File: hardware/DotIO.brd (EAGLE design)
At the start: 30 x 65 mm, 37 parts, among them CN1 1X4-BIG, U1 ATMEGA328P-MU-QFN32, X1 S4B-ZR, X2 S4B-ZR, X3 S4B-ZR, X4 S4B-ZR, X5 S4B-ZR, X6 S4B-ZR, X7 S4B-ZR

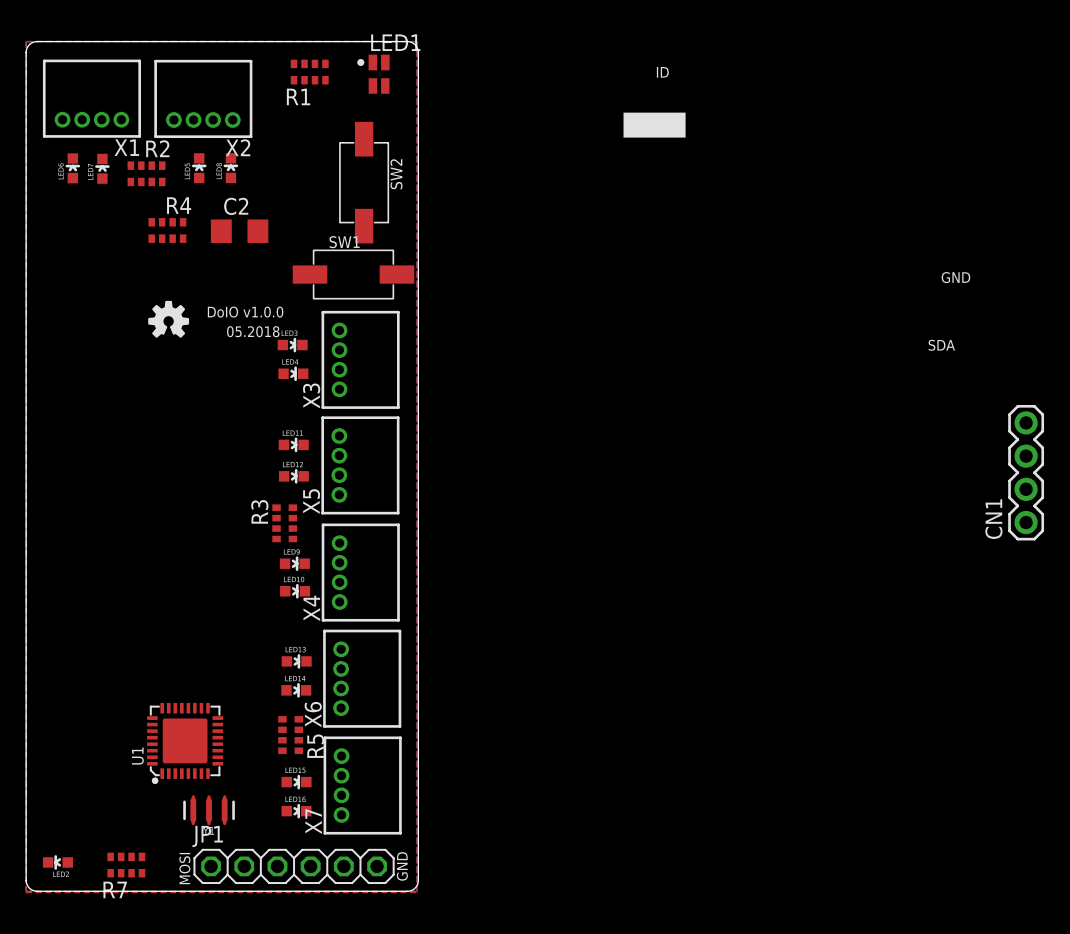
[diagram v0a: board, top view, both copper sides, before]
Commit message: Initial routing
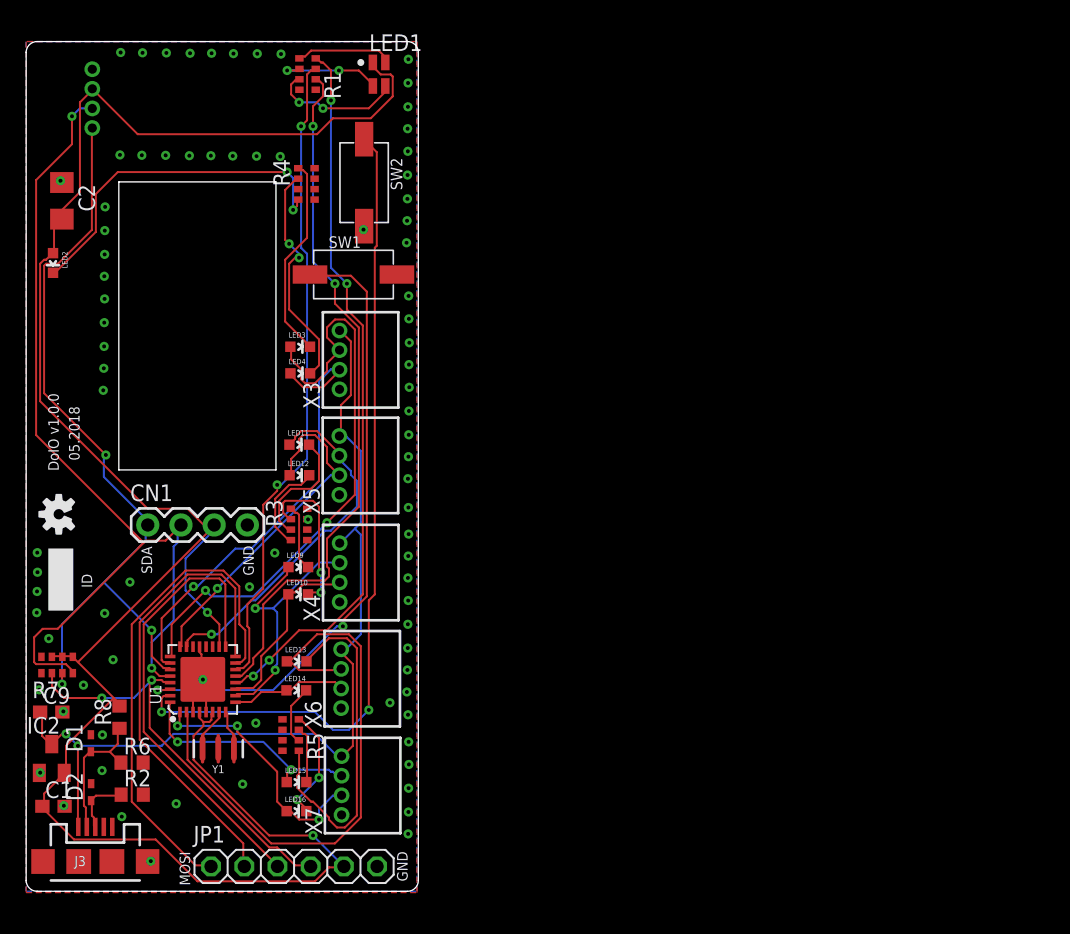
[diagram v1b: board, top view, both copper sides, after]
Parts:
- removed LED5, LED6, LED7, LED8: (no value), SparkFun:LED-0603
- removed X2: S4B-ZR, con-jst:S4B-ZR
- added C1, C9: 1uF, rcl:C0603
- added D1, D2: (no value), diode:SOD523
- added IC2: (no value), MCP1700:SOT-23
- added J3: USB-MICROB, SparkFun-Retired:USB-MICROB
- added R6: 68Ω, rcl:R0603
- added R8: 1.5kΩ, rcl:R0603
- R2: value 150Ω -> 68Ω; device SparkFun:0603-ARV -> rcl:R0603
- moved CN1 67.2 mm to (9.30, 28.0), turned to 0 degrees
- moved R2 47.5 mm to (8.12, 7.39), turned to 0 degrees
- moved LED2 45.9 mm to (2.06, 48.1), turned to 180 degrees
- moved LOGO1 17.0 mm to (2.50, 28.8), turned to 90 degrees
- moved R7 16.2 mm to (2.37, 17.3)
- moved C2 13.8 mm to (2.73, 52.8), turned to 270 degrees
- moved R4 11.2 mm to (21.4, 54.1), turned to 270 degrees
- moved U1 4.90 mm to (13.5, 16.2)
- moved Y1 4.76 mm to (14.7, 10.9)
- moved X1 1.62 mm to (5.06, 60.6), flipped to the bottom, turned to 90 degrees
- moved R3 1.10 mm to (20.9, 28.1)
- moved LED3 0.59 mm to (21.0, 41.7)
- moved LED4 0.53 mm to (21.0, 39.6)
- moved LED12 0.43 mm to (20.9, 31.8)
- moved LED11 0.42 mm to (20.9, 34.2)
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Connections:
- net LED renamed RGB_RED
- removed net ADCENA: U1.13
- removed net CS_FLASH: U1.23
- removed net N$11: LED6.C, R2.1
- removed net N$12: LED7.C, R2.2
- removed net N$13: LED8.C, R2.4
- removed net N$3: LED5.C, R2.3
- removed net OUTA: LED11.A, LED3.A, LED5.A, LED6.A, U1.14, X1.3, X2.3, X3.3, X5.3
- removed net OUTB: LED12.A, LED4.A, LED7.A, LED8.A, X1.2, X2.2, X3.2, X5.2
- removed net RSEL: U1.26
- removed net RXD: R1.3
- removed net TXD: R1.2
- new net 4_0: LED11.A, U1.23, X5.3
- new net 4_1: LED12.A, U1.24, X5.2
- new net 5_0: LED3.A, U1.25, X3.3
- new net 5_1: LED4.A, U1.26, X3.2
- new net RGB_BLUE: R1.3, U1.14
- new net RGB_GREEN: R1.2, U1.13
- new net USB_D+: D2.C, J3.D+, R2.1
- new net USB_D-: D1.C, J3.D-, R6.1, R8.1
- net +3V3: now also C1.1, IC2.2, R8.2, X1.3
- net +5V: now also C9.1, IC2.3, J3.VBUS; no longer X1.4, X2.4
- net D+: now also R2.2; no longer U1.25
- net D-: now also R6.2; no longer U1.24
- net GND: now also C1.2, C9.2, D1.A, D2.A, IC2.1, J3.GND, J3.MT1, J3.MT2, X1.4; no longer R2.5, R2.6, R2.7, R2.8, X1.1, X2.1
- net SCL: now also X1.2
- net SDA: now also X1.1
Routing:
- net +3V3: track 0.00 -> 162.6 mm, vias 0 -> 2
- net SCL: track 0.00 -> 72.6 mm, vias 0 -> 2
- net +5V: track 0.00 -> 70.9 mm, vias 0 -> 2
- net PUSH_RIGHT: track 0.00 -> 63.1 mm, vias 0 -> 2
- net SDA: track 0.00 -> 60.6 mm, vias 0 -> 3
- net RGB_RED: track 0.00 -> 55.2 mm, vias 0 -> 4
- net RGB_GREEN: track 0.00 -> 53.7 mm, vias 0 -> 2
- net RGB_BLUE: track 0.00 -> 49.6 mm, vias 0 -> 2
- net PUSH_UP: track 0.00 -> 48.4 mm, vias 0 -> 2
- net 5_0: track 0.00 -> 45.9 mm, vias 0 -> 2
- net 2_0: track 0.00 -> 45.0 mm
- net MOSI: track 0.00 -> 38.7 mm
- net MISO: track 0.00 -> 36.5 mm
- net SCK: track 0.00 -> 35.4 mm
- net 5_1: track 0.00 -> 34.8 mm, vias 0 -> 1
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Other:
- outline, holes or cut-outs redrawn
